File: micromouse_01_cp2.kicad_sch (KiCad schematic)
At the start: 36 parts, among them IC2 MPU-6500, IC5 DRV8835DSSR, M1 MK06-4.5, M2 MK06-4.5, U10 MA730, U11 MA730, U13 MCP3464T-E/NC, U9 ESP32-S3-PICO-1-N8R2

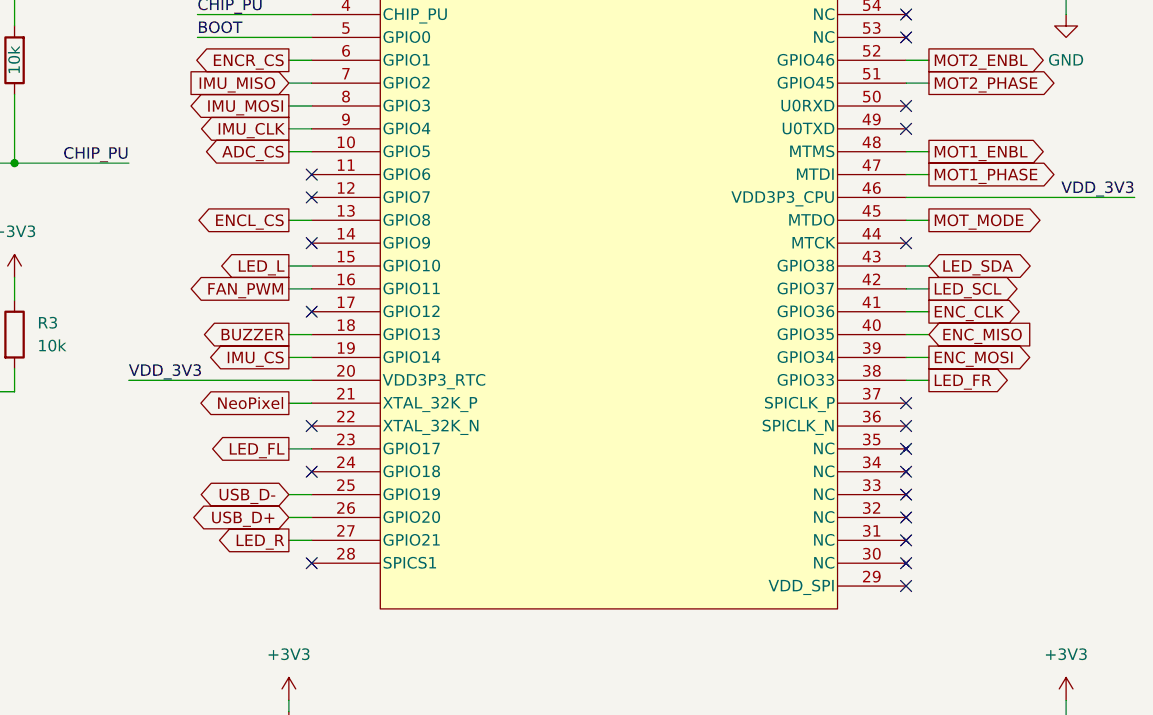
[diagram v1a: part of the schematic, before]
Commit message: N8R8用回路（仮）
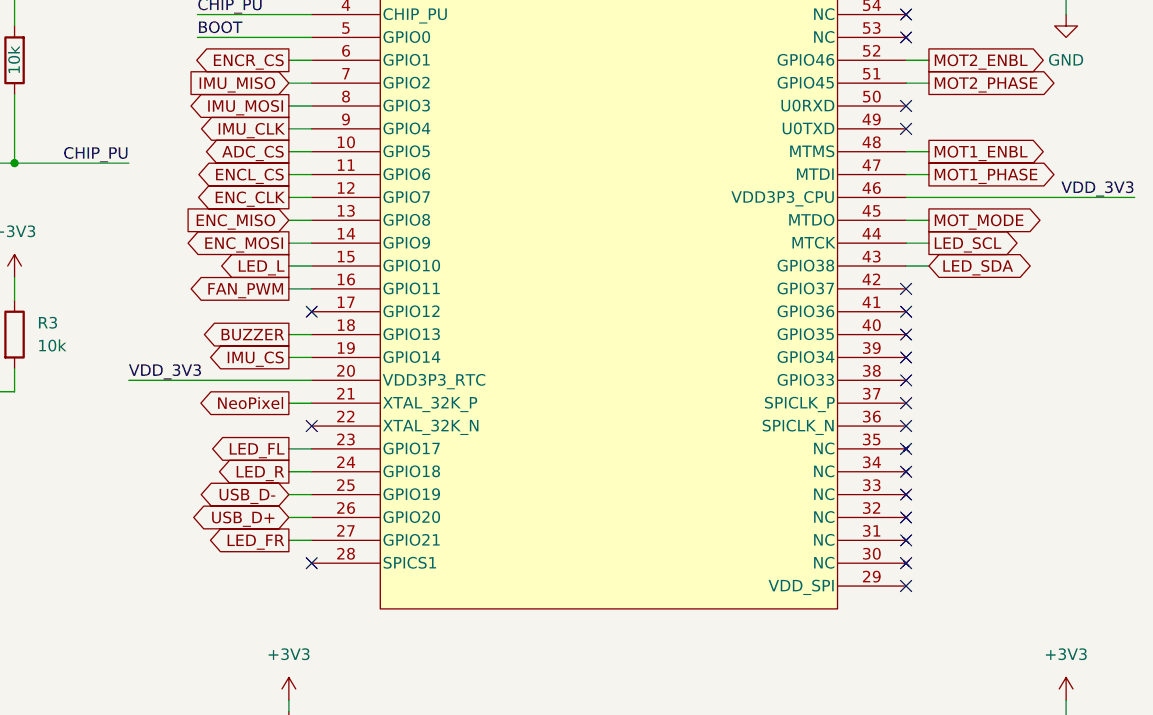
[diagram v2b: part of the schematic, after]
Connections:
- net ENCL_CS: now also U9.11 (GPIO6); no longer U9.13 (GPIO8)
- net ENC_CLK: now also U9.12 (GPIO7); no longer U9.41 (GPIO36)
- net ENC_MISO: now also U9.13 (GPIO8); no longer U9.40 (GPIO35)
- net ENC_MOSI: now also U9.14 (GPIO9); no longer U9.39 (GPIO34)
- net LED_FR: now also U9.27 (GPIO21); no longer U9.38 (GPIO33)
- net LED_R: now also U9.24 (GPIO18); no longer U9.27 (GPIO21)
- net LED_SCL: now also U9.44 (MTCK); no longer U9.42 (GPIO37)
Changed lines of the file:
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@@
   (no_connect (at 256.54 86.36))
   (no_connect (at 73.66 137.16))
+  (no_connect (at 256.54 76.2))
   (no_connect (at 121.92 45.72))
-  (no_connect (at 256.54 66.04))
-  (no_connect (at 190.5 91.44))
+  (no_connect (at 256.54 73.66))
   (no_connect (at 256.54 40.64))
   (no_connect (at 68.58 106.68))
   (no_connect (at 96.52 43.18))
-  (no_connect (at 190.5 66.04))
   (no_connect (at 60.96 137.16))
   (no_connect (at 71.12 40.64))
@@
   (no_connect (at 71.12 33.02))
   (no_connect (at 71.12 137.16))
+  (no_connect (at 256.54 71.12))
   (no_connect (at 256.54 43.18))
   (no_connect (at 238.76 142.24))
@@
   (no_connect (at 190.5 73.66))
   (no_connect (at 63.5 137.16))
+  (no_connect (at 256.54 78.74))
   (no_connect (at 38.1 119.38))
-  (no_connect (at 190.5 58.42))
   (no_connect (at 256.54 101.6))
   (no_connect (at 48.26 76.2))
@@
   (no_connect (at 121.92 30.48))
   (no_connect (at 256.54 88.9))
-  (no_connect (at 190.5 60.96))
+  (no_connect (at 256.54 81.28))
   (no_connect (at 121.92 40.64))
   (no_connect (at 71.12 106.68))
@@
     (stroke (width 0) (type default))
   )
-  (wire (pts (xy 259.08 76.2) (xy 256.54 76.2))
-    (stroke (width 0) (type default))
-  )
   (wire (pts (xy 109.22 53.34) (xy 109.22 55.88))
     (stroke (width 0) (type default))
@@
     (stroke (width 0) (type default))
   )
-  (wire (pts (xy 259.08 78.74) (xy 256.54 78.74))
-    (stroke (width 0) (type default))
-  )
   (wire (pts (xy 128.27 180.34) (xy 128.27 184.15))
     (stroke (width 0) (type default))
@@
     (stroke (width 0) (type default))
   )
-  (wire (pts (xy 259.08 71.12) (xy 256.54 71.12))
-    (stroke (width 0) (type default))
-  )
   (wire (pts (xy 170.18 132.08) (xy 170.18 143.51))
     (stroke (width 0) (type default))
@@
     (stroke (width 0) (type default))
   )
+  (wire (pts (xy 187.96 91.44) (xy 190.5 91.44))
+    (stroke (width 0) (type default))
+  )
   (wire (pts (xy 30.48 68.58) (xy 30.48 71.12))
     (stroke (width 0) (type default))
@@
     (stroke (width 0) (type default))
   )
+  (wire (pts (xy 187.96 58.42) (xy 190.5 58.42))
+    (stroke (width 0) (type default))
+  )
   (wire (pts (xy 101.6 124.46) (xy 96.52 124.46))
     (stroke (width 0) (type default))
@@
     (stroke (width 0) (type default))
   )
+  (wire (pts (xy 187.96 66.04) (xy 190.5 66.04))
+    (stroke (width 0) (type default))
+  )
   (wire (pts (xy 76.2 22.86) (xy 73.66 22.86))
     (stroke (width 0) (type default))
@@
     (stroke (width 0) (type default))
   )
-  (wire (pts (xy 259.08 81.28) (xy 256.54 81.28))
-    (stroke (width 0) (type default))
-  )
   (wire (pts (xy 58.42 50.8) (xy 58.42 53.34))
     (stroke (width 0) (type default))
@@
     (stroke (width 0) (type default))
   )
+  (wire (pts (xy 256.54 66.04) (xy 259.08 66.04))
+    (stroke (width 0) (type default))
+  )
   (wire (pts (xy 157.48 57.15) (xy 170.18 57.15))
     (stroke (width 0) (type default))
@@
     (stroke (width 0) (type default))
   )
+  (wire (pts (xy 187.96 60.96) (xy 190.5 60.96))
+    (stroke (width 0) (type default))
+  )
   (wire (pts (xy 82.55 102.87) (xy 83.82 102.87))
     (stroke (width 0) (type default))
@@
   )
   (wire (pts (xy 161.29 175.26) (xy 161.29 177.8))
-    (stroke (width 0) (type default))
-  )
-  (wire (pts (xy 259.08 73.66) (xy 256.54 73.66))
     (stroke (width 0) (type default))
   )
@@
     )
   )
+  (global_label "ENC_MOSI" (shape output) (at 187.96 66.04 180) (fields_autoplaced)
+    (effects (font (size 1.27 1.27)) (justify right))
+    (property "Intersheetrefs" "${INTERSHEET_REFS}" (at 175.6615 66.04 0)
+      (effects (font (size 1.27 1.27)) (justify right) hide)
+    )
+  )
   (global_label "LED_SDA" (shape bidirectional) (at 259.08 68.58 0) (fields_autoplaced)
     (effects (font (size 1.27 1.27)) (justify left))
@@
     )
   )
-  (global_label "ENC_MOSI" (shape output) (at 259.08 78.74 0) (fields_autoplaced)
-    (effects (font (size 1.27 1.27)) (justify left))
-    (property "Intersheetrefs" "${INTERSHEET_REFS}" (at 271.3785 78.74 0)
-      (effects (font (size 1.27 1.27)) (justify left) hide)
+  (global_label "ENC_MISO" (shape input) (at 187.96 63.5 180) (fields_autoplaced)
+    (effects (font (size 1.27 1.27)) (justify right))
+    (property "Intersheetrefs" "${INTERSHEET_REFS}" (at 175.6615 63.5 0)
+      (effects (font (size 1.27 1.27)) (justify right) hide)
     )
   )
@@
     )
   )
-  (global_label "ENCL_CS" (shape output) (at 187.96 63.5 180) (fields_autoplaced)
-    (effects (font (size 1.27 1.27)) (justify right))
-    (property "Intersheetrefs" "${INTERSHEET_REFS}" (at 176.7501 63.5 0)
-      (effects (font (size 1.27 1.27)) (justify right) hide)
-    )
-  )
   (global_label "ENCR_CS" (shape input) (at 93.98 38.1 180) (fields_autoplaced)
     (effects (font (size 1.27 1.27)) (justify right))
@@
     )
   )
+  (global_label "ENC_CLK" (shape output) (at 187.96 60.96 180) (fields_autoplaced)
+    (effects (font (size 1.27 1.27)) (justify right))
+    (property "Intersheetrefs" "${INTERSHEET_REFS}" (at 176.6896 60.96 0)
+      (effects (font (size 1.27 1.27)) (justify right) hide)
+    )
+  )
   (global_label "SENS_L" (shape input) (at 167.64 139.7 180) (fields_autoplaced)
     (effects (font (size 1.27 1.27)) (justify right))
@@
     )
   )
+  (global_label "LED_SCL" (shape output) (at 259.08 66.04 0) (fields_autoplaced)
+    (effects (font (size 1.27 1.27)) (justify left))
+    (property "Intersheetrefs" "${INTERSHEET_REFS}" (at 269.9875 66.04 0)
+      (effects (font (size 1.27 1.27)) (justify left) hide)
+    )
+  )
   (global_label "LED_FL" (shape output) (at 187.96 88.9 180) (fields_autoplaced)
     (effects (font (size 1.27 1.27)) (justify right))
@@
     )
   )
-  (global_label "ENC_MISO" (shape input) (at 259.08 76.2 0) (fields_autoplaced)
-    (effects (font (size 1.27 1.27)) (justify left))
-    (property "Intersheetrefs" "${INTERSHEET_REFS}" (at 271.3785 76.2 0)
-      (effects (font (size 1.27 1.27)) (justify left) hide)
-    )
-  )
   (global_label "ENC_MISO" (shape output) (at 43.18 33.02 180) (fields_autoplaced)
     (effects (font (size 1.27 1.27)) (justify right))
@@
     )
   )
-  (global_label "LED_SCL" (shape output) (at 259.08 71.12 0) (fields_autoplaced)
-    (effects (font (size 1.27 1.27)) (justify left))
-    (property "Intersheetrefs" "${INTERSHEET_REFS}" (at 269.9875 71.12 0)
-      (effects (font (size 1.27 1.27)) (justify left) hide)
+  (global_label "LED_FR" (shape output) (at 187.96 99.06 180) (fields_autoplaced)
+    (effects (font (size 1.27 1.27)) (justify right))
+    (property "Intersheetrefs" "${INTERSHEET_REFS}" (at 178.2015 99.06 0)
+      (effects (font (size 1.27 1.27)) (justify right) hide)
     )
   )
@@
     )
   )
-  (global_label "LED_FR" (shape output) (at 259.08 81.28 0) (fields_autoplaced)
-    (effects (font (size 1.27 1.27)) (justify left))
-    (property "Intersheetrefs" "${INTERSHEET_REFS}" (at 268.8385 81.28 0)
-      (effects (font (size 1.27 1.27)) (justify left) hide)
+  (global_label "ENCL_CS" (shape output) (at 187.96 58.42 180) (fields_autoplaced)
+    (effects (font (size 1.27 1.27)) (justify right))
+    (property "Intersheetrefs" "${INTERSHEET_REFS}" (at 176.7501 58.42 0)
+      (effects (font (size 1.27 1.27)) (justify right) hide)
     )
   )
@@
     )
   )
-  (global_label "ENC_CLK" (shape output) (at 259.08 73.66 0) (fields_autoplaced)
-    (effects (font (size 1.27 1.27)) (justify left))
-    (property "Intersheetrefs" "${INTERSHEET_REFS}" (at 270.3504 73.66 0)
-      (effects (font (size 1.27 1.27)) (justify left) hide)
-    )
-  )
   (global_label "ADC_CS" (shape input) (at 241.3 152.4 0) (fields_autoplaced)
     (effects (font (size 1.27 1.27)) (justify left))
@@
     )
   )
-  (global_label "LED_R" (shape output) (at 187.96 99.06 180) (fields_autoplaced)
-    (effects (font (size 1.27 1.27)) (justify right))
-    (property "Intersheetrefs" "${INTERSHEET_REFS}" (at 179.2901 99.06 0)
-      (effects (font (size 1.27 1.27)) (justify right) hide)
-    )
-  )
   (global_label "MOT1_PHASE" (shape output) (at 259.08 58.42 0) (fields_autoplaced)
     (effects (font (size 1.27 1.27)) (justify left))
@@
     )
   )
+  (global_label "LED_R" (shape output) (at 187.96 91.44 180) (fields_autoplaced)
+    (effects (font (size 1.27 1.27)) (justify right))
+    (property "Intersheetrefs" "${INTERSHEET_REFS}" (at 179.2901 91.44 0)
+      (effects (font (size 1.27 1.27)) (justify right) hide)
+    )
+  )
